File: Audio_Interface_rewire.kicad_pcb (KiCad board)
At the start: 2 copper layers, 62 parts, among them IC1 REG103GA-3.3_2K5, IC2 PCM2906CDB, IC3 INA849DGKT, J1 USB_B_Micro, J2 SJ-435107RS, J3 Vol. knob1 22k, J4 Vol. knob2 22k, J5 SW_PUSH_3PDT, J6 External mic. conn., Q1 J304, SW1 HID0, SW2 HID1, SW3 HID2, U1 NMA0515SC, Y1 12MHz

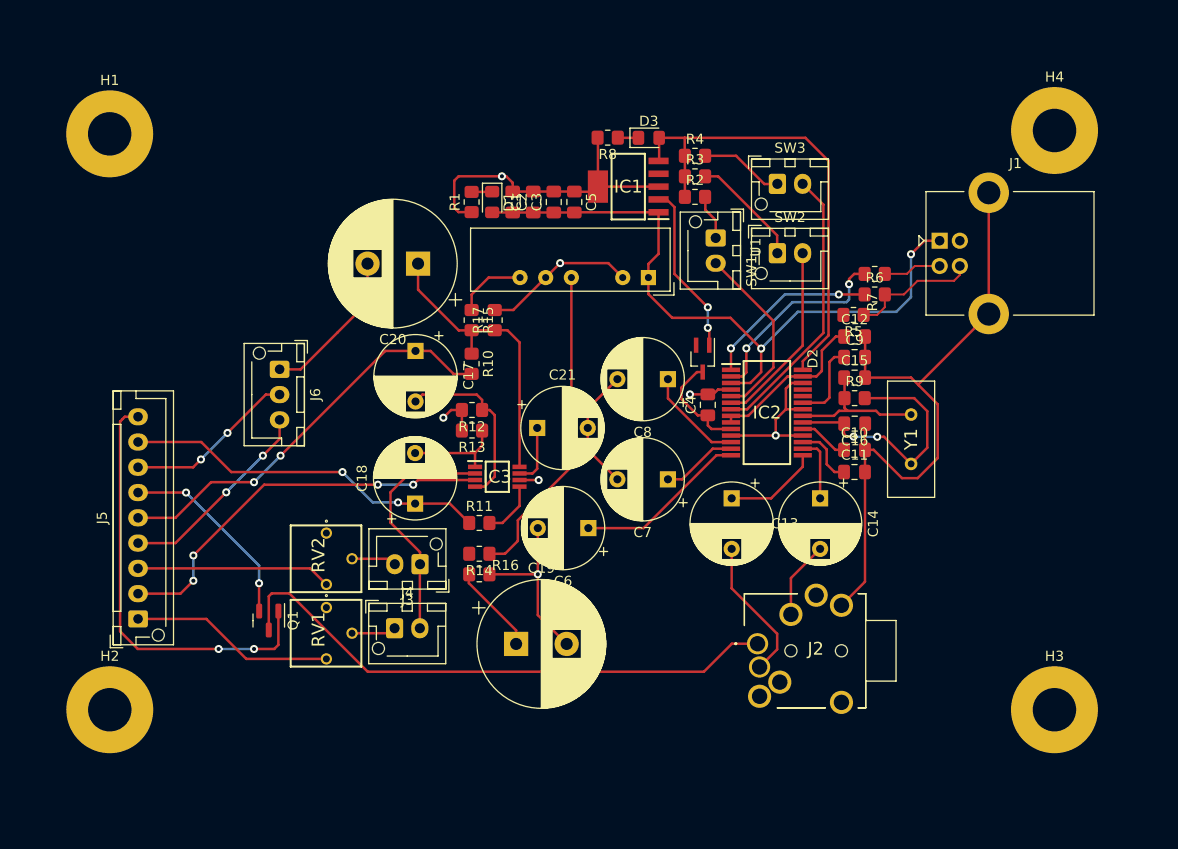
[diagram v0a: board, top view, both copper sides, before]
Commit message: Reviewed Gnorins work
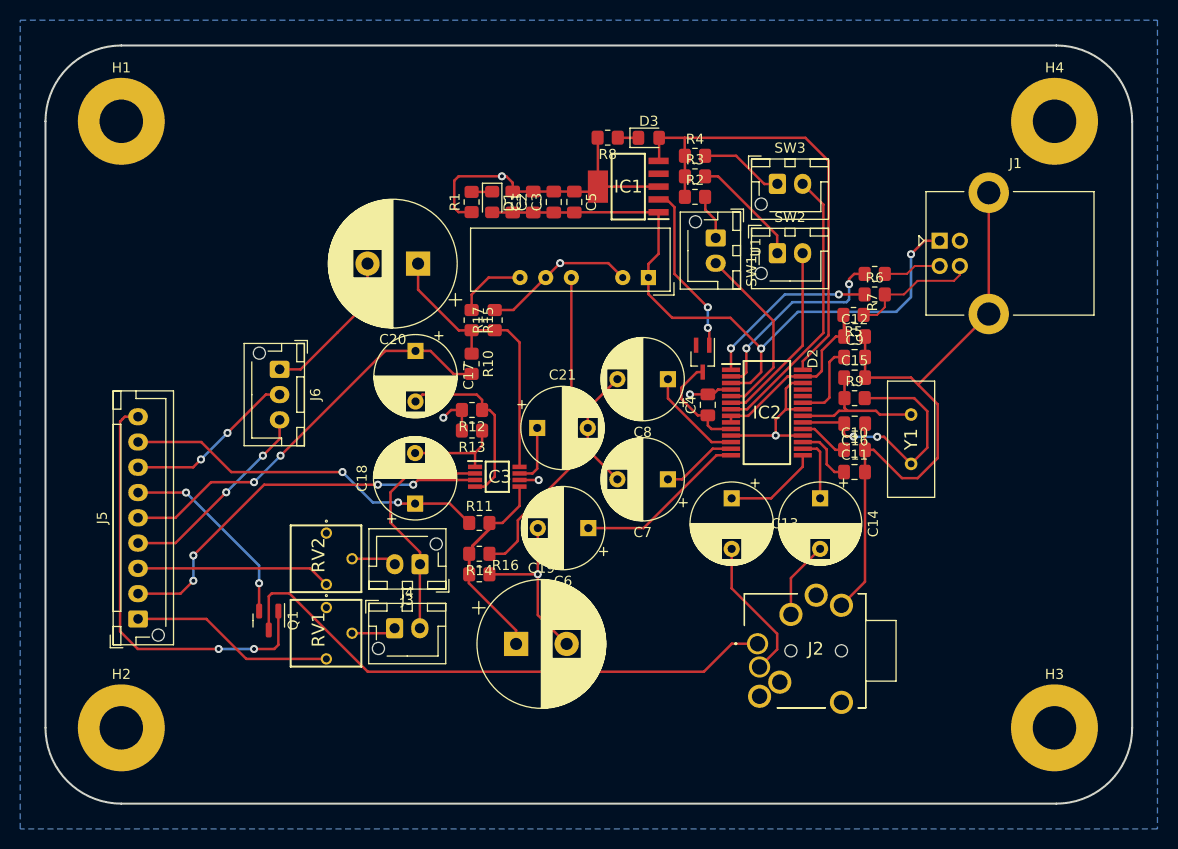
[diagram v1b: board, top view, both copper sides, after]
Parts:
- moved H2 2.12 mm to (97.5, 130.0)
- moved H3 1.79 mm to (189.8, 130.0)
- moved H1 1.69 mm to (97.5, 70.0)
- moved H4 0.91 mm to (189.8, 70.0)
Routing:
- net /-vs: track 14.4 -> 20.3 mm
- net /VDDI: track 16.3 -> 18.4 mm
- added copper zone on B.Cu, net GND
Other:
- board outline added: 107.5 x 75 mm
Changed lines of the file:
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@@
   )
   (footprint "MountingHole:MountingHole_4.3mm_M4_Pad" (layer "F.Cu")
-    (at 189.82 70.91)
+    (at 189.82 70)
     (descr "Mounting Hole 4.3mm, M4")
     (tags "mounting hole 4.3mm m4")
@@
   )
   (footprint "MountingHole:MountingHole_4.3mm_M4_Pad" (layer "F.Cu")
-    (at 189.812 128.21)
+    (at 189.812 130)
     (descr "Mounting Hole 4.3mm, M4")
     (tags "mounting hole 4.3mm m4")
@@
   )
   (footprint "MountingHole:MountingHole_4.3mm_M4_Pad" (layer "F.Cu")
-    (at 96.35 71.24)
+    (at 97.5 70)
     (descr "Mounting Hole 4.3mm, M4")
     (tags "mounting hole 4.3mm m4")
@@
   )
   (footprint "MountingHole:MountingHole_4.3mm_M4_Pad" (layer "F.Cu")
-    (at 96.36 128.21)
+    (at 97.5 130)
     (descr "Mounting Hole 4.3mm, M4")
     (tags "mounting hole 4.3mm m4")
@@
     )
   )
+  (gr_line (start 190 62.5) (end 97.5 62.5) (layer "Edge.Cuts") (width 0.2))
+  (gr_arc (start 97.5 137.5) (mid 92.196699 135.303301) (end 90 130) (layer "Edge.Cuts") (width 0.2))
+  (gr_line (start 190 137.5) (end 97.5 137.5) (layer "Edge.Cuts") (width 0.2))
+  (gr_arc (start 190 62.5) (mid 195.303301 64.696699) (end 197.5 70) (layer "Edge.Cuts") (width 0.2))
+  (gr_arc (start 90 70) (mid 92.196699 64.696699) (end 97.5 62.5) (layer "Edge.Cuts") (width 0.2))
+  (gr_arc (start 197.5 130) (mid 195.303301 135.303301) (end 190 137.5) (layer "Edge.Cuts") (width 0.2))
+  (gr_line (start 197.5 130) (end 197.5 70) (layer "Edge.Cuts") (width 0.2))
+  (gr_line (start 90 70) (end 90 130) (layer "Edge.Cuts") (width 0.2))
   (segment (start 134.1985 79.0215) (end 134.186 79.009) (width 0.25) (layer "F.Cu") (net 1))
   (segment (start 136.218 79.0215) (end 134.1985 79.0215) (width 0.25) (layer "F.Cu") (net 1))
@@
   (segment (start 168.19 91.29) (end 166.8 92.68) (width 0.25) (layer "F.Cu") (net 12))
   (segment (start 157.814 99.787) (end 157.814 99.137) (width 0.25) (layer "F.Cu") (net 12))
+  (segment (start 169.0045 89.2245) (end 168.934 89.154) (width 0.3) (layer "F.Cu") (net 12))
   (segment (start 166.263 95.237) (end 164.914 95.237) (width 0.25) (layer "F.Cu") (net 12))
   (segment (start 166.8 94.7) (end 166.263 95.237) (width 0.25) (layer "F.Cu") (net 12))
   (segment (start 166.8 92.68) (end 166.8 94.7) (width 0.25) (layer "F.Cu") (net 12))
   (segment (start 169.0045 91.29) (end 168.19 91.29) (width 0.25) (layer "F.Cu") (net 12))
+  (segment (start 169.0045 91.29) (end 169.0045 89.2245) (width 0.3) (layer "F.Cu") (net 12))
   (segment (start 166.63 107.297349) (end 166.63 102.7) (width 0.25) (layer "F.Cu") (net 13))
   (segment (start 166.63 102.7) (end 166.317 102.387) (width 0.25) (layer "F.Cu") (net 13))
@@
   (segment (start 132.465349 102.818651) (end 132.494 102.79) (width 0.25) (layer "F.Cu") (net 20))
   (segment (start 126.566 102.818651) (end 132.465349 102.818651) (width 0.25) (layer "F.Cu") (net 20))
+  (segment (start 131.916 114.814) (end 131.916 112.782) (width 0.3) (layer "F.Cu") (net 21))
   (segment (start 131.88 115.68) (end 131.88 114.85) (width 0.25) (layer "F.Cu") (net 21))
+  (segment (start 133.916 110.334) (end 133.916 109.734) (width 0.3) (layer "F.Cu") (net 21))
   (segment (start 136.556041 121.7) (end 136.556041 120.356041) (width 0.25) (layer "F.Cu") (net 21))
+  (segment (start 131.916 112.782) (end 132.25 112.448) (width 0.3) (layer "F.Cu") (net 21))
   (segment (start 136.894 106.137) (end 136.894 108.042) (width 0.25) (layer "F.Cu") (net 21))
+  (segment (start 132.25 112) (end 133.916 110.334) (width 0.3) (layer "F.Cu") (net 21))
   (segment (start 136.556041 120.356041) (end 131.88 115.68) (width 0.25) (layer "F.Cu") (net 21))
   (segment (start 131.88 114.85) (end 131.916 114.814) (width 0.25) (layer "F.Cu") (net 21))
+  (segment (start 132.25 112.448) (end 132.25 112) (width 0.3) (layer "F.Cu") (net 21))
   (segment (start 136.894 108.042) (end 135.202 109.734) (width 0.25) (layer "F.Cu") (net 21))
   (segment (start 135.202 109.734) (end 133.916 109.734) (width 0.25) (layer "F.Cu") (net 21))
@@
   (via (at 107.13 122.2) (size 0.8) (drill 0.4) (layers "F.Cu" "B.Cu") (net 62))
   (segment (start 107.13 122.2) (end 110.63 122.2) (width 0.25) (layer "B.Cu") (net 62))
+  (zone (net 2) (net_name "GND") (layer "B.Cu") (hatch edge 0.508)
+    (connect_pads (clearance 0.508))
+    (min_thickness 0.254) (filled_areas_thickness no)
+    (fill yes (thermal_gap 0.508) (thermal_bridge_width 0.508))
+    (polygon
+      (pts
+        (xy 200 140)
+        (xy 87.5 140)
+        (xy 87.5 60)
+        (xy 200 60)
+      )
+    )
+  )
 )
